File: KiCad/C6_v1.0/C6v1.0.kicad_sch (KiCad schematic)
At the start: 4 parts

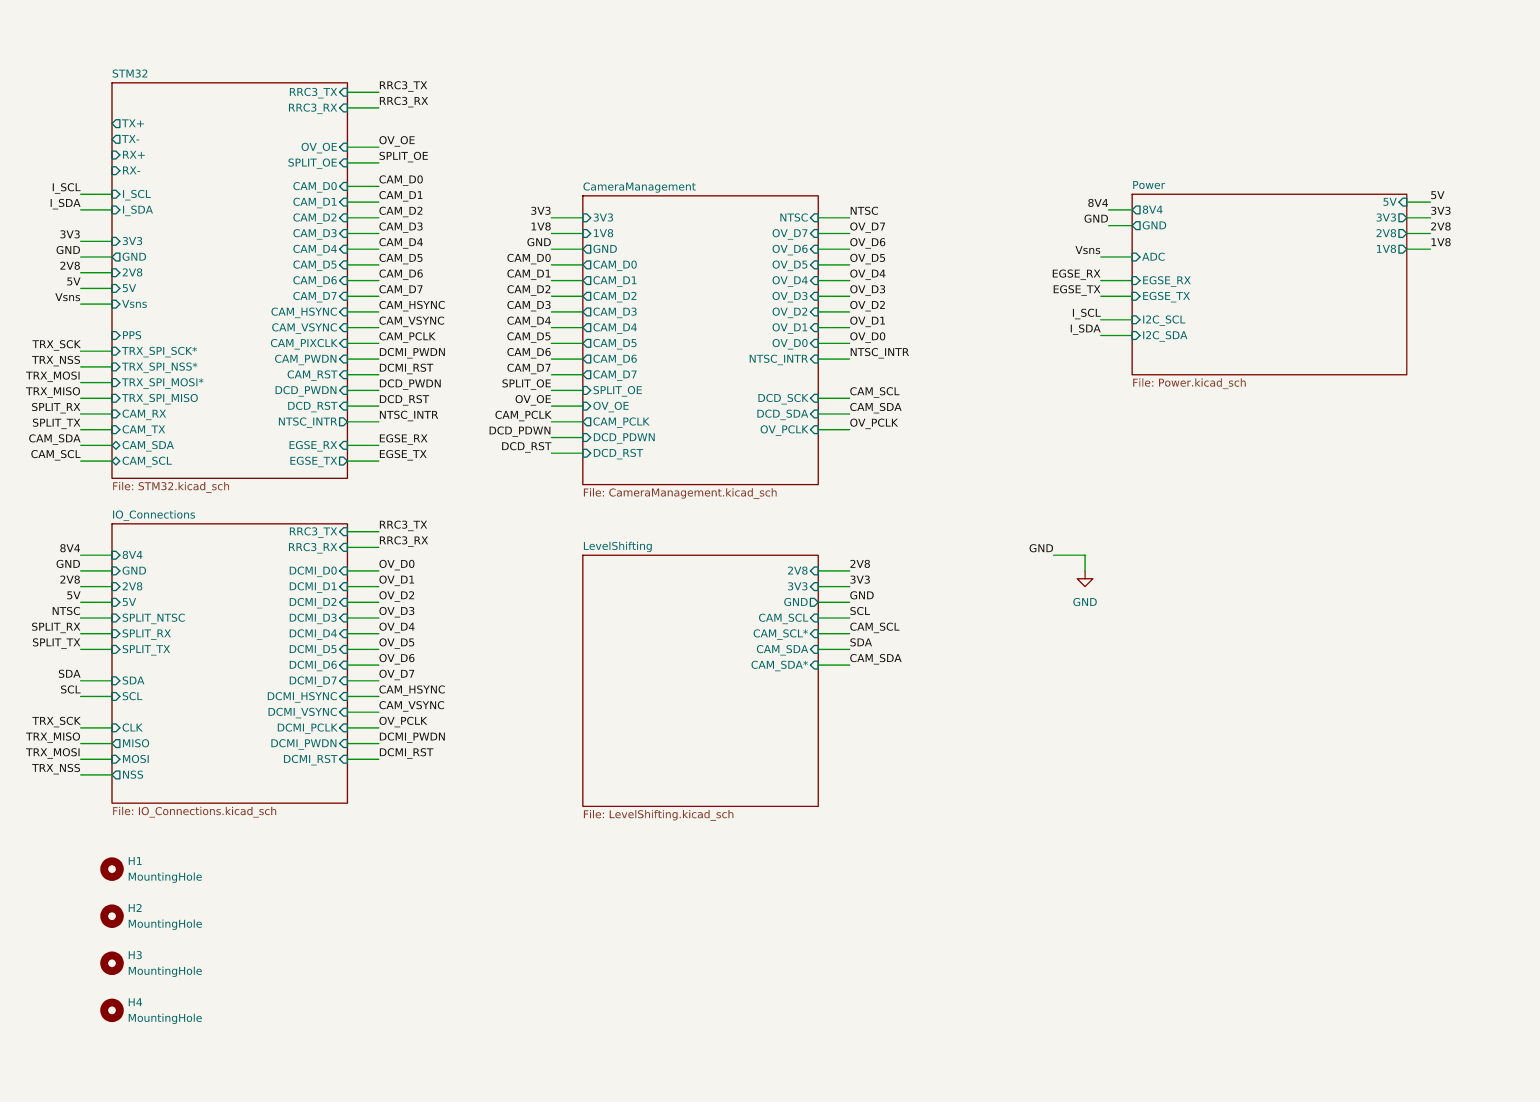
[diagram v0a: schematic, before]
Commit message: DCMI1-Me0
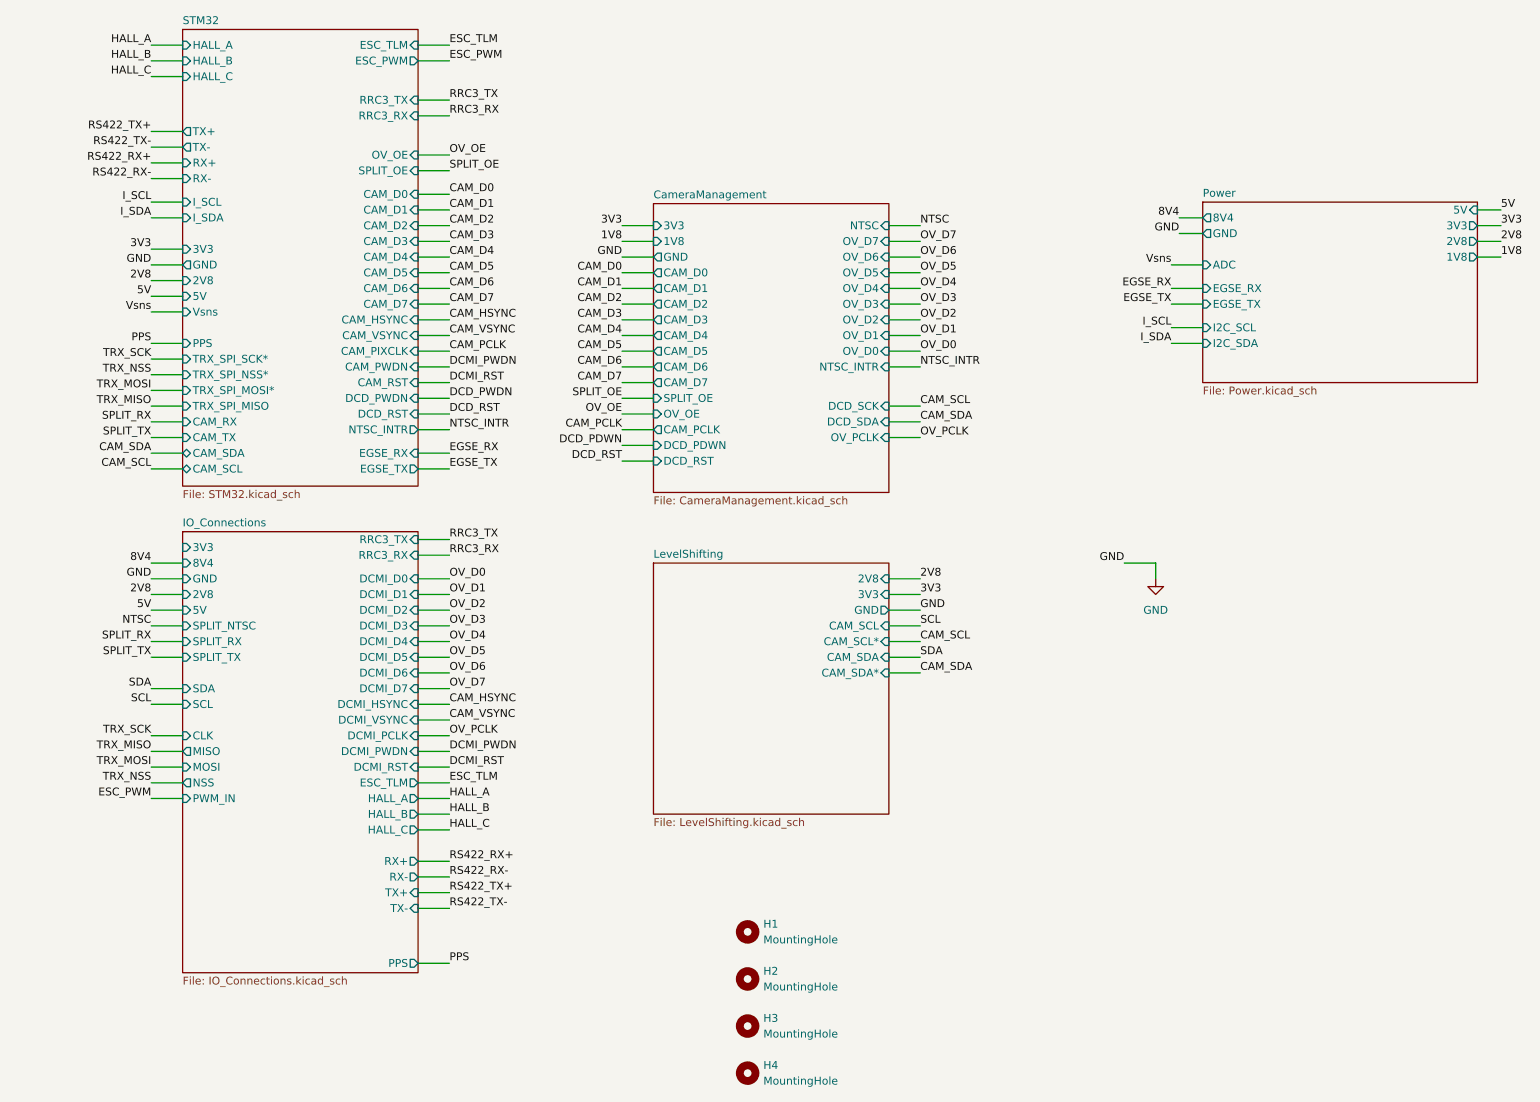
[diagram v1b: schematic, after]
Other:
- sheet IO_Connections ports: added 3V3, ESC_TLM, HALL_A, HALL_B, HALL_C, PPS, PWM_IN, RX+, RX-, TX+, TX-; removed none
- sheet STM32 ports: added ESC_PWM, ESC_TLM, HALL_A, HALL_B, HALL_C; removed none
- moved on the sheet: H1, H2, H3, H4
